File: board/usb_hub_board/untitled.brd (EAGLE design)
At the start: 11.2 x 23.9 mm, 12 parts

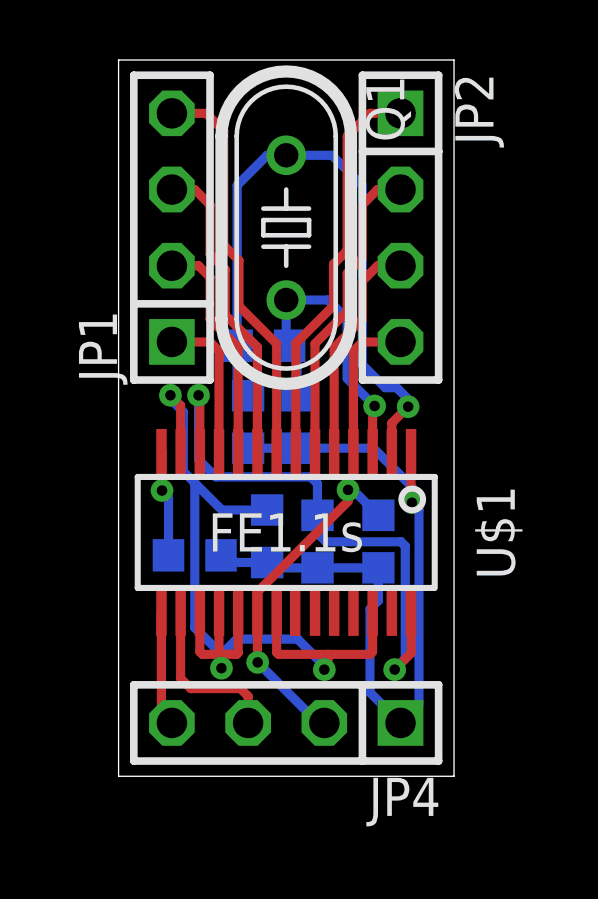
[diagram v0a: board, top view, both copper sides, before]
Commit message: Revert "Merge remote-tracking branch 'origin/Develop' into feature_#37"
This reverts commit cb103155361e8766478c6830db153463370c0739, reversing
changes made to 84e093fe944e1f8653a6822ff34e6f8740617cb5.
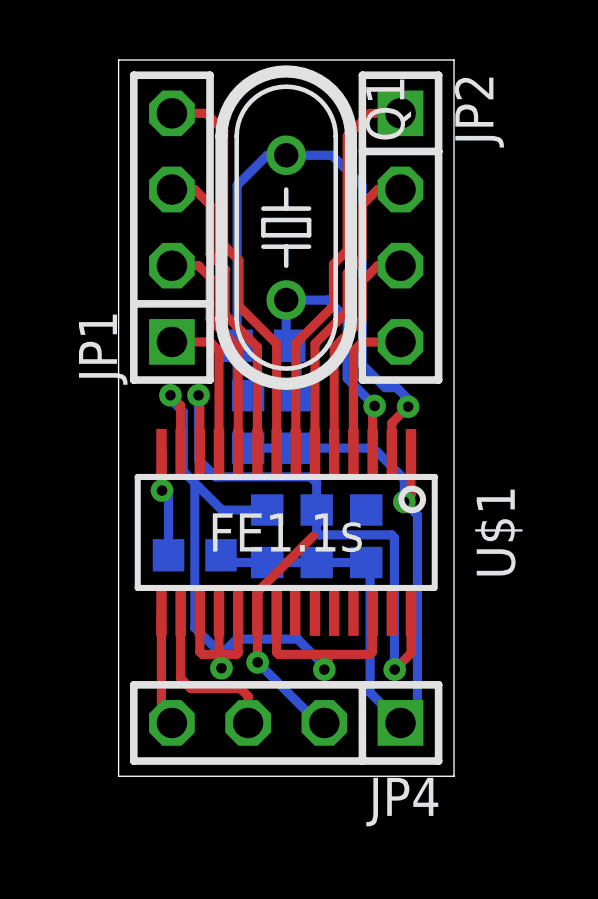
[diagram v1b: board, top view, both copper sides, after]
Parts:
- moved C3 0.44 mm to (8.26, 8.00)
- moved C2 0.18 mm to (6.60, 8.00)
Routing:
- net +5V: track 11.4 -> 8.18 mm, vias 2 -> 1
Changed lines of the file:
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@@
 <?xml version="1.0" encoding="utf-8"?>
 <!DOCTYPE eagle SYSTEM "eagle.dtd">
-<eagle version="9.6.2">
+<eagle version="9.6.1">
 <drawing>
 <settings>
@@
 <attribute name="VALUE" x="3.303" y="7.201" size="1.016" layer="28" rot="MR90"/>
 </element>
-<element name="C2" library="generic" package="SMD1608" value="" x="6.6294" y="7.8232" smashed="yes" rot="MR90">
-<attribute name="NAME" x="7.2794" y="7.0232" size="1.016" layer="26" rot="MR90"/>
-<attribute name="VALUE" x="4.9794" y="7.0232" size="1.016" layer="28" rot="MR90"/>
-</element>
-<element name="C3" library="generic" package="SMD1608" value="" x="8.6614" y="7.8232" smashed="yes" rot="MR270">
-<attribute name="NAME" x="8.0114" y="8.6232" size="1.016" layer="26" rot="MR270"/>
-<attribute name="VALUE" x="10.3114" y="8.6232" size="1.016" layer="28" rot="MR270"/>
+<element name="C2" library="generic" package="SMD1608" value="" x="6.604" y="8.001" smashed="yes" rot="MR90">
+<attribute name="NAME" x="7.254" y="7.201" size="1.016" layer="26" rot="MR90"/>
+<attribute name="VALUE" x="4.954" y="7.201" size="1.016" layer="28" rot="MR90"/>
+</element>
+<element name="C3" library="generic" package="SMD1608" value="" x="8.255" y="8.001" smashed="yes" rot="MR270">
+<attribute name="NAME" x="7.605" y="8.801" size="1.016" layer="26" rot="MR270"/>
+<attribute name="VALUE" x="9.905" y="8.801" size="1.016" layer="28" rot="MR270"/>
 </element>
 <element name="C4" library="generic" package="SMD1608" value="" x="4.318" y="11.811" smashed="yes" rot="MR90">
@@
 <wire x1="2.665" y1="12.7" x2="2.665" y2="10.55458125" width="0.3048" layer="16"/>
 <wire x1="3.24038125" y1="9.9792" x2="2.665" y2="10.55458125" width="0.3048" layer="16"/>
-<wire x1="6.6294" y1="8.6982" x2="6.6294" y2="9.7536" width="0.3048" layer="16"/>
-<wire x1="6.6294" y1="9.7536" x2="6.4038" y2="9.9792" width="0.3048" layer="16"/>
+<wire x1="6.604" y1="8.876" x2="6.604" y2="9.779" width="0.3048" layer="16"/>
+<wire x1="6.604" y1="9.779" x2="6.4038" y2="9.9792" width="0.3048" layer="16"/>
 <wire x1="6.4038" y1="9.9792" x2="3.24038125" y2="9.9792" width="0.3048" layer="16"/>
 <wire x1="9.748" y1="5.428" x2="9.748" y2="4.101" width="0.3048" layer="1"/>
 <wire x1="9.748" y1="4.101" x2="9.203" y2="3.556" width="0.3048" layer="1"/>
 <via x="9.203" y="3.556" extent="1-16" drill="0.35"/>
-<wire x1="9.1948" y1="3.5642" x2="9.203" y2="3.556" width="0.3048" layer="16"/>
-<wire x1="6.6294" y1="8.1026" x2="6.6294" y2="8.6982" width="0.3048" layer="16"/>
-<wire x1="6.9144" y1="7.8176" x2="6.6294" y2="8.1026" width="0.3048" layer="16"/>
-<wire x1="9.41505" y1="7.8176" x2="6.9144" y2="7.8176" width="0.3048" layer="16"/>
-<wire x1="9.5558" y1="7.67685" x2="9.41505" y2="7.8176" width="0.3048" layer="16"/>
-<wire x1="9.5558" y1="3.9252" x2="9.1948" y2="3.5642" width="0.3048" layer="16"/>
-<wire x1="9.5558" y1="7.67685" x2="9.5558" y2="3.9252" width="0.3048" layer="16"/>
+<wire x1="9.1948" y1="7.9502" x2="9.1948" y2="3.5642" width="0.3048" layer="16"/>
+<wire x1="9.203" y1="3.556" x2="9.1948" y2="3.5642" width="0.3048" layer="16"/>
+<wire x1="9.1948" y1="7.9502" x2="9.0988" y2="8.0462" width="0.3048" layer="16"/>
+<wire x1="6.604" y1="8.128" x2="6.604" y2="8.876" width="0.3048" layer="16"/>
+<wire x1="6.6858" y1="8.0462" x2="6.604" y2="8.128" width="0.3048" layer="16"/>
+<wire x1="9.0988" y1="8.0462" x2="6.6858" y2="8.0462" width="0.3048" layer="16"/>
 </signal>
 <signal name="N$5">
@@
 <wire x1="4.953" y1="7.126" x2="3.937" y2="7.126" width="0.3048" layer="16"/>
 <wire x1="3.937" y1="7.126" x2="3.415" y2="7.366" width="0.3048" layer="16"/>
+<wire x1="6.604" y1="7.126" x2="4.953" y2="7.126" width="0.3048" layer="16"/>
 <wire x1="5.969" y1="10.936" x2="8.495" y2="10.936" width="0.3048" layer="16"/>
-<wire x1="8.495" y1="10.936" x2="9.779" y2="9.652" width="0.3048" layer="16"/>
-<wire x1="9.779" y1="9.652" x2="9.779" y2="9.1186" width="0.3048" layer="16"/>
-<wire x1="9.748" y1="10.828" x2="9.748" y2="9.1496" width="0.3048" layer="1"/>
-<wire x1="9.748" y1="9.1496" x2="9.779" y2="9.1186" width="0.3048" layer="1"/>
-<via x="9.779" y="9.1186" extent="1-16" drill="0.35"/>
-<wire x1="9.779" y1="9.1186" x2="10.013" y2="8.8846" width="0.3048" layer="16"/>
-<wire x1="10.013" y1="2.393" x2="9.398" y2="1.778" width="0.3048" layer="16"/>
-<wire x1="10.013" y1="8.8846" x2="10.013" y2="2.393" width="0.3048" layer="16"/>
-<wire x1="8.6614" y1="6.9482" x2="8.6614" y2="5.856" width="0.3048" layer="16"/>
-<wire x1="8.6614" y1="5.856" x2="8.382" y2="5.5766" width="0.3048" layer="16"/>
+<wire x1="8.495" y1="10.936" x2="9.525" y2="9.906" width="0.3048" layer="16"/>
+<wire x1="9.525" y1="9.906" x2="9.525" y2="9.144" width="0.3048" layer="16"/>
+<wire x1="9.748" y1="10.828" x2="9.748" y2="9.367" width="0.3048" layer="1"/>
+<wire x1="9.748" y1="9.367" x2="9.525" y2="9.144" width="0.3048" layer="1"/>
+<via x="9.525" y="9.144" extent="1-16" drill="0.35"/>
+<wire x1="6.604" y1="7.126" x2="8.255" y2="7.126" width="0.3048" layer="16"/>
+<wire x1="9.525" y1="9.144" x2="9.9622" y2="8.7068" width="0.3048" layer="16"/>
+<wire x1="9.9622" y1="2.3422" x2="9.398" y2="1.778" width="0.3048" layer="16"/>
+<wire x1="9.9622" y1="8.7068" x2="9.9622" y2="2.3422" width="0.3048" layer="16"/>
+<wire x1="8.255" y1="7.126" x2="8.382" y2="6.999" width="0.3048" layer="16"/>
 <wire x1="8.382" y1="2.794" x2="9.398" y2="1.778" width="0.3048" layer="16"/>
-<wire x1="8.382" y1="5.5766" x2="8.382" y2="2.794" width="0.3048" layer="16"/>
-<wire x1="4.953" y1="7.126" x2="5.1308" y2="6.9482" width="0.3048" layer="16"/>
-<wire x1="5.1308" y1="6.9482" x2="6.6294" y2="6.9482" width="0.3048" layer="16"/>
-<wire x1="6.6294" y1="6.9482" x2="8.6614" y2="6.9482" width="0.3048" layer="16"/>
+<wire x1="8.382" y1="6.999" x2="8.382" y2="2.794" width="0.3048" layer="16"/>
 </signal>
 <signal name="+5V">
@@
 <contactref element="U$1" pad="20"/>
 <contactref element="JP4" pad="2"/>
-<wire x1="4.628" y1="6.14405" x2="4.628" y2="5.428" width="0.3048" layer="1"/>
+<wire x1="8.396" y1="8.876" x2="8.255" y2="8.876" width="0.3048" layer="16"/>
+<wire x1="4.628" y1="5.428" x2="4.628" y2="6.14405" width="0.3048" layer="1"/>
+<wire x1="4.628" y1="6.14405" x2="6.48495" y2="8.001" width="0.3048" layer="1"/>
 <wire x1="4.628" y1="5.428" x2="4.628" y2="3.8040875" width="0.3048" layer="1"/>
 <wire x1="4.628" y1="3.8040875" x2="4.6355" y2="3.7965875" width="0.3048" layer="1"/>
@@
 <wire x1="4.6355" y1="3.7965875" x2="6.6540875" y2="1.778" width="0.3048" layer="16"/>
 <wire x1="6.6540875" y1="1.778" x2="6.858" y2="1.778" width="0.3048" layer="16"/>
-<wire x1="8.6614" y1="8.6982" x2="7.8122" y2="9.5474" width="0.3048" layer="16"/>
-<wire x1="7.6492" y1="9.5474" x2="7.8122" y2="9.5474" width="0.3048" layer="16"/>
-<via x="7.6492" y="9.5474" extent="1-16" drill="0.35" diameter="0.65"/>
-<wire x1="7.6492" y1="9.5474" x2="7.6492" y2="9.16525" width="0.3048" layer="1"/>
-<wire x1="7.6492" y1="9.16525" x2="4.628" y2="6.14405" width="0.3048" layer="1"/>
+<wire x1="6.48495" y1="8.001" x2="8.255" y2="8.876" width="0" layer="19" extent="1-16"/>
 </signal>
 <signal name="N$11">

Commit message: エラー解消
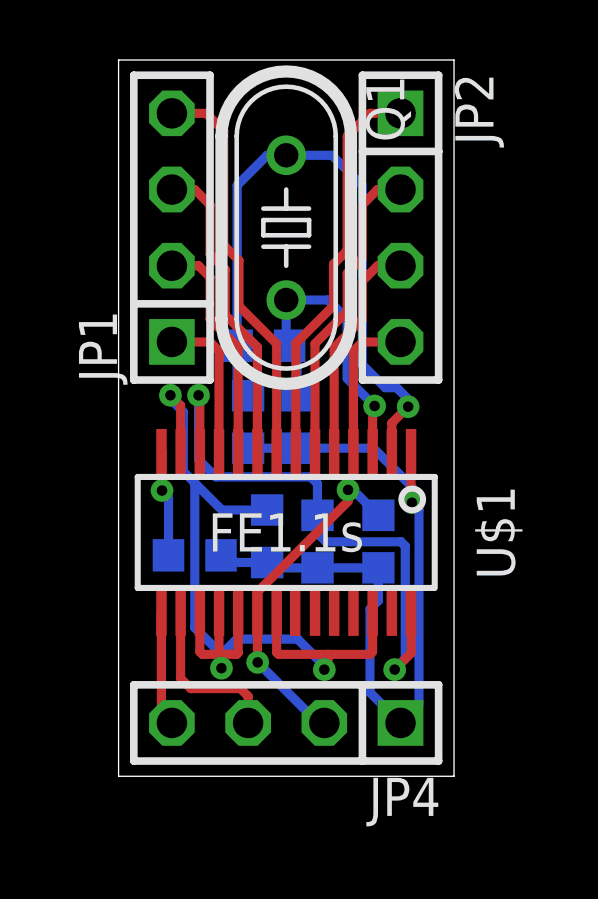
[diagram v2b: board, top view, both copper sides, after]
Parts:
- moved C3 0.44 mm to (8.66, 7.82)
- moved C2 0.18 mm to (6.63, 7.82)
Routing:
- net +5V: track 8.18 -> 11.4 mm, vias 1 -> 2
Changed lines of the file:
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@@
 <?xml version="1.0" encoding="utf-8"?>
 <!DOCTYPE eagle SYSTEM "eagle.dtd">
-<eagle version="9.6.1">
+<eagle version="9.6.2">
 <drawing>
 <settings>
@@
 <attribute name="VALUE" x="3.303" y="7.201" size="1.016" layer="28" rot="MR90"/>
 </element>
-<element name="C2" library="generic" package="SMD1608" value="" x="6.604" y="8.001" smashed="yes" rot="MR90">
-<attribute name="NAME" x="7.254" y="7.201" size="1.016" layer="26" rot="MR90"/>
-<attribute name="VALUE" x="4.954" y="7.201" size="1.016" layer="28" rot="MR90"/>
-</element>
-<element name="C3" library="generic" package="SMD1608" value="" x="8.255" y="8.001" smashed="yes" rot="MR270">
-<attribute name="NAME" x="7.605" y="8.801" size="1.016" layer="26" rot="MR270"/>
-<attribute name="VALUE" x="9.905" y="8.801" size="1.016" layer="28" rot="MR270"/>
+<element name="C2" library="generic" package="SMD1608" value="" x="6.6294" y="7.8232" smashed="yes" rot="MR90">
+<attribute name="NAME" x="7.2794" y="7.0232" size="1.016" layer="26" rot="MR90"/>
+<attribute name="VALUE" x="4.9794" y="7.0232" size="1.016" layer="28" rot="MR90"/>
+</element>
+<element name="C3" library="generic" package="SMD1608" value="" x="8.6614" y="7.8232" smashed="yes" rot="MR270">
+<attribute name="NAME" x="8.0114" y="8.6232" size="1.016" layer="26" rot="MR270"/>
+<attribute name="VALUE" x="10.3114" y="8.6232" size="1.016" layer="28" rot="MR270"/>
 </element>
 <element name="C4" library="generic" package="SMD1608" value="" x="4.318" y="11.811" smashed="yes" rot="MR90">
@@
 <wire x1="2.665" y1="12.7" x2="2.665" y2="10.55458125" width="0.3048" layer="16"/>
 <wire x1="3.24038125" y1="9.9792" x2="2.665" y2="10.55458125" width="0.3048" layer="16"/>
-<wire x1="6.604" y1="8.876" x2="6.604" y2="9.779" width="0.3048" layer="16"/>
-<wire x1="6.604" y1="9.779" x2="6.4038" y2="9.9792" width="0.3048" layer="16"/>
+<wire x1="6.6294" y1="8.6982" x2="6.6294" y2="9.7536" width="0.3048" layer="16"/>
+<wire x1="6.6294" y1="9.7536" x2="6.4038" y2="9.9792" width="0.3048" layer="16"/>
 <wire x1="6.4038" y1="9.9792" x2="3.24038125" y2="9.9792" width="0.3048" layer="16"/>
 <wire x1="9.748" y1="5.428" x2="9.748" y2="4.101" width="0.3048" layer="1"/>
 <wire x1="9.748" y1="4.101" x2="9.203" y2="3.556" width="0.3048" layer="1"/>
 <via x="9.203" y="3.556" extent="1-16" drill="0.35"/>
-<wire x1="9.1948" y1="7.9502" x2="9.1948" y2="3.5642" width="0.3048" layer="16"/>
-<wire x1="9.203" y1="3.556" x2="9.1948" y2="3.5642" width="0.3048" layer="16"/>
-<wire x1="9.1948" y1="7.9502" x2="9.0988" y2="8.0462" width="0.3048" layer="16"/>
-<wire x1="6.604" y1="8.128" x2="6.604" y2="8.876" width="0.3048" layer="16"/>
-<wire x1="6.6858" y1="8.0462" x2="6.604" y2="8.128" width="0.3048" layer="16"/>
-<wire x1="9.0988" y1="8.0462" x2="6.6858" y2="8.0462" width="0.3048" layer="16"/>
+<wire x1="9.1948" y1="3.5642" x2="9.203" y2="3.556" width="0.3048" layer="16"/>
+<wire x1="6.6294" y1="8.1026" x2="6.6294" y2="8.6982" width="0.3048" layer="16"/>
+<wire x1="6.9144" y1="7.8176" x2="6.6294" y2="8.1026" width="0.3048" layer="16"/>
+<wire x1="9.41505" y1="7.8176" x2="6.9144" y2="7.8176" width="0.3048" layer="16"/>
+<wire x1="9.5558" y1="7.67685" x2="9.41505" y2="7.8176" width="0.3048" layer="16"/>
+<wire x1="9.5558" y1="3.9252" x2="9.1948" y2="3.5642" width="0.3048" layer="16"/>
+<wire x1="9.5558" y1="7.67685" x2="9.5558" y2="3.9252" width="0.3048" layer="16"/>
 </signal>
 <signal name="N$5">
@@
 <wire x1="4.953" y1="7.126" x2="3.937" y2="7.126" width="0.3048" layer="16"/>
 <wire x1="3.937" y1="7.126" x2="3.415" y2="7.366" width="0.3048" layer="16"/>
-<wire x1="6.604" y1="7.126" x2="4.953" y2="7.126" width="0.3048" layer="16"/>
 <wire x1="5.969" y1="10.936" x2="8.495" y2="10.936" width="0.3048" layer="16"/>
-<wire x1="8.495" y1="10.936" x2="9.525" y2="9.906" width="0.3048" layer="16"/>
-<wire x1="9.525" y1="9.906" x2="9.525" y2="9.144" width="0.3048" layer="16"/>
-<wire x1="9.748" y1="10.828" x2="9.748" y2="9.367" width="0.3048" layer="1"/>
-<wire x1="9.748" y1="9.367" x2="9.525" y2="9.144" width="0.3048" layer="1"/>
-<via x="9.525" y="9.144" extent="1-16" drill="0.35"/>
-<wire x1="6.604" y1="7.126" x2="8.255" y2="7.126" width="0.3048" layer="16"/>
-<wire x1="9.525" y1="9.144" x2="9.9622" y2="8.7068" width="0.3048" layer="16"/>
-<wire x1="9.9622" y1="2.3422" x2="9.398" y2="1.778" width="0.3048" layer="16"/>
-<wire x1="9.9622" y1="8.7068" x2="9.9622" y2="2.3422" width="0.3048" layer="16"/>
-<wire x1="8.255" y1="7.126" x2="8.382" y2="6.999" width="0.3048" layer="16"/>
+<wire x1="8.495" y1="10.936" x2="9.779" y2="9.652" width="0.3048" layer="16"/>
+<wire x1="9.779" y1="9.652" x2="9.779" y2="9.1186" width="0.3048" layer="16"/>
+<wire x1="9.748" y1="10.828" x2="9.748" y2="9.1496" width="0.3048" layer="1"/>
+<wire x1="9.748" y1="9.1496" x2="9.779" y2="9.1186" width="0.3048" layer="1"/>
+<via x="9.779" y="9.1186" extent="1-16" drill="0.35"/>
+<wire x1="9.779" y1="9.1186" x2="10.013" y2="8.8846" width="0.3048" layer="16"/>
+<wire x1="10.013" y1="2.393" x2="9.398" y2="1.778" width="0.3048" layer="16"/>
+<wire x1="10.013" y1="8.8846" x2="10.013" y2="2.393" width="0.3048" layer="16"/>
+<wire x1="8.6614" y1="6.9482" x2="8.6614" y2="5.856" width="0.3048" layer="16"/>
+<wire x1="8.6614" y1="5.856" x2="8.382" y2="5.5766" width="0.3048" layer="16"/>
 <wire x1="8.382" y1="2.794" x2="9.398" y2="1.778" width="0.3048" layer="16"/>
-<wire x1="8.382" y1="6.999" x2="8.382" y2="2.794" width="0.3048" layer="16"/>
+<wire x1="8.382" y1="5.5766" x2="8.382" y2="2.794" width="0.3048" layer="16"/>
+<wire x1="4.953" y1="7.126" x2="5.1308" y2="6.9482" width="0.3048" layer="16"/>
+<wire x1="5.1308" y1="6.9482" x2="6.6294" y2="6.9482" width="0.3048" layer="16"/>
+<wire x1="6.6294" y1="6.9482" x2="8.6614" y2="6.9482" width="0.3048" layer="16"/>
 </signal>
 <signal name="+5V">
@@
 <contactref element="U$1" pad="20"/>
 <contactref element="JP4" pad="2"/>
-<wire x1="8.396" y1="8.876" x2="8.255" y2="8.876" width="0.3048" layer="16"/>
-<wire x1="4.628" y1="5.428" x2="4.628" y2="6.14405" width="0.3048" layer="1"/>
-<wire x1="4.628" y1="6.14405" x2="6.48495" y2="8.001" width="0.3048" layer="1"/>
+<wire x1="4.628" y1="6.14405" x2="4.628" y2="5.428" width="0.3048" layer="1"/>
 <wire x1="4.628" y1="5.428" x2="4.628" y2="3.8040875" width="0.3048" layer="1"/>
 <wire x1="4.628" y1="3.8040875" x2="4.6355" y2="3.7965875" width="0.3048" layer="1"/>
@@
 <wire x1="4.6355" y1="3.7965875" x2="6.6540875" y2="1.778" width="0.3048" layer="16"/>
 <wire x1="6.6540875" y1="1.778" x2="6.858" y2="1.778" width="0.3048" layer="16"/>
-<wire x1="6.48495" y1="8.001" x2="8.255" y2="8.876" width="0" layer="19" extent="1-16"/>
+<wire x1="8.6614" y1="8.6982" x2="7.8122" y2="9.5474" width="0.3048" layer="16"/>
+<wire x1="7.6492" y1="9.5474" x2="7.8122" y2="9.5474" width="0.3048" layer="16"/>
+<via x="7.6492" y="9.5474" extent="1-16" drill="0.35" diameter="0.65"/>
+<wire x1="7.6492" y1="9.5474" x2="7.6492" y2="9.16525" width="0.3048" layer="1"/>
+<wire x1="7.6492" y1="9.16525" x2="4.628" y2="6.14405" width="0.3048" layer="1"/>
 </signal>
 <signal name="N$11">
